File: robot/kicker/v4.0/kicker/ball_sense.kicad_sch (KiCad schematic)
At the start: 4 parts, among them J10 SM08B-GHS-TB

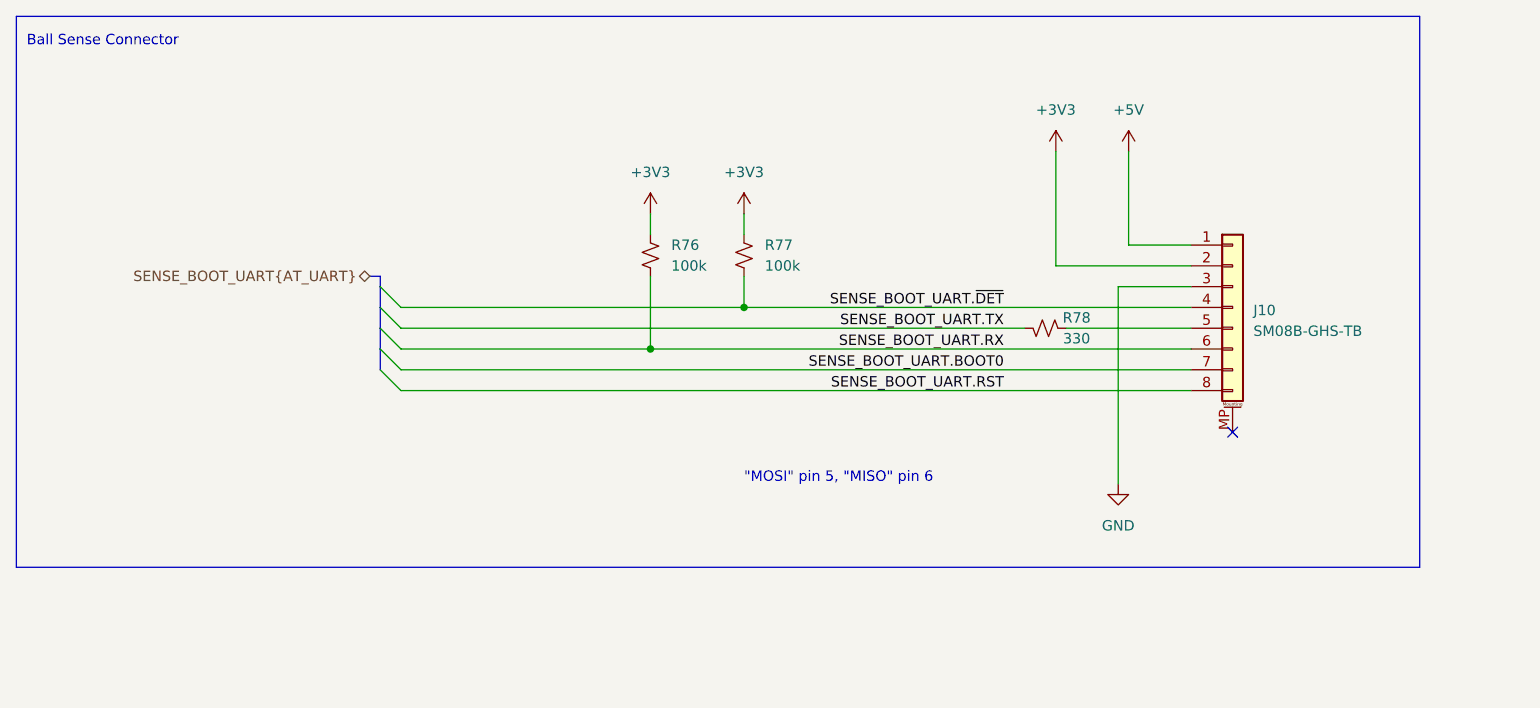
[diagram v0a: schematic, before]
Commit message: fixed old conenctors
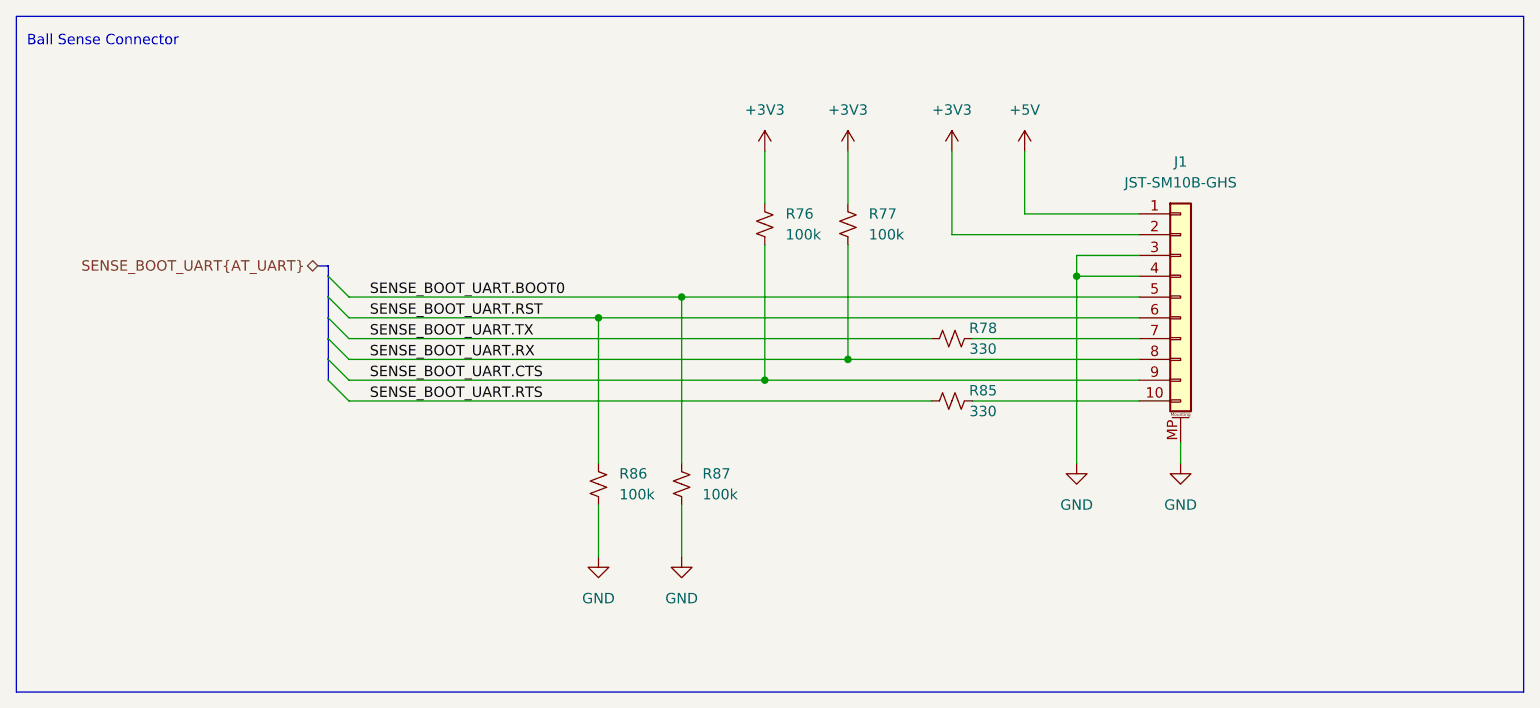
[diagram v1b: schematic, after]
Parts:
- removed J10: SM08B-GHS-TB, Connector_JST:JST_GH_SM08B-GHS-TB_1x08-1MP_P1.25mm_Horizontal, symbol Connector_Generic_MountingPin:Conn_01x08_MountingPin
- added J1: JST-SM10B-GHS, Connector_JST:JST_GH_SM10B-GHS-TB_1x10-1MP_P1.25mm_Horizontal, symbol Connector_Generic_MountingPin:Conn_01x10_MountingPin
- added R85: 330, Resistor_SMD:R_0402_1005Metric, symbol Device:R_Small_US
- added R86, R87: 100k, Resistor_SMD:R_0402_1005Metric, symbol Device:R_Small_US
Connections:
- net SENSE_BOOT_UART.~{DET} is gone; now on net SENSE_BOOT_UART.RX: R77.2
- net +3V3: now also J1.2 (Pin_2)
- net +5V: now also J1.1 (Pin_1)
- net GND: now also J1.3 (Pin_3), J1.4 (Pin_4), J1.MP (MountPin), R86.2, R87.2
- net SENSE_BOOT_UART.BOOT0: now also J1.5 (Pin_5), R87.1
- net SENSE_BOOT_UART.RST: now also J1.6 (Pin_6), R86.1
- net SENSE_BOOT_UART.RX: now also J1.8 (Pin_8); no longer R76.2
- net SENSE_BOOT_UART.TX: now also R78.1; no longer R78.2
- new net: J1.7 (Pin_7), R78.2
- new net: J1.10 (Pin_10), R85.2
- new net SENSE_BOOT_UART.CTS: J1.9 (Pin_9), R76.2
- new net SENSE_BOOT_UART.RTS: R85.1
- no-connect marks 1 -> 0
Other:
- note removed: ""MOSI" pin 5, "MISO" pin 6"

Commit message: kicker v4.0 prod files
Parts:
- J1: LCSC (none) -> C2683602
- R76, R77, R86, R87: LCSC (none) -> C60491
- R78, R85: LCSC (none) -> C105875
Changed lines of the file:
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@@
+			)
+		)
+		(property "LCSC" "C105875"
+			(at 137.16 57.15 0)
+			(effects
+				(font
+					(size 1.27 1.27)
+				)
+				(hide yes)
 			)
 		)
@@
 			)
 		)
+		(property "LCSC" "C60491"
+			(at 92.71 74.9299 0)
+			(effects
+				(font
+					(size 1.27 1.27)
+				)
+				(hide yes)
+			)
+		)
 		(pin "1"
 		)
@@
 			)
 		)
+		(property "LCSC" "C60491"
+			(at 102.87 74.9299 0)
+			(effects
+				(font
+					(size 1.27 1.27)
+				)
+				(hide yes)
+			)
+		)
 		(pin "1"
 		)
@@
 			)
 		)
+		(property "LCSC" "C60491"
+			(at 113.03 43.1799 0)
+			(effects
+				(font
+					(size 1.27 1.27)
+				)
+				(hide yes)
+			)
+		)
 		(pin "1"
 		)
@@
 			)
 		)
+		(property "LCSC" "C105875"
+			(at 137.16 64.77 0)
+			(effects
+				(font
+					(size 1.27 1.27)
+				)
+				(hide yes)
+			)
+		)
 		(pin "1"
 		)
@@
 			)
 		)
+		(property "LCSC" "C2683602"
+			(at 161.29 36.83 0)
+			(effects
+				(font
+					(size 1.27 1.27)
+				)
+				(hide yes)
+			)
+		)
 		(pin "8"
 		)
@@
 			(effects
 				(font
+					(size 1.27 1.27)
+				)
+				(hide yes)
+			)
+		)
+		(property "LCSC" "C60491"
+			(at 123.19 43.1799 0)
+			(effects
+				(font
